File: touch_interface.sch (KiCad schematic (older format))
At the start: 18 parts, among them SW2 SW_Push, U5 ASMT-YTC2-0AA02

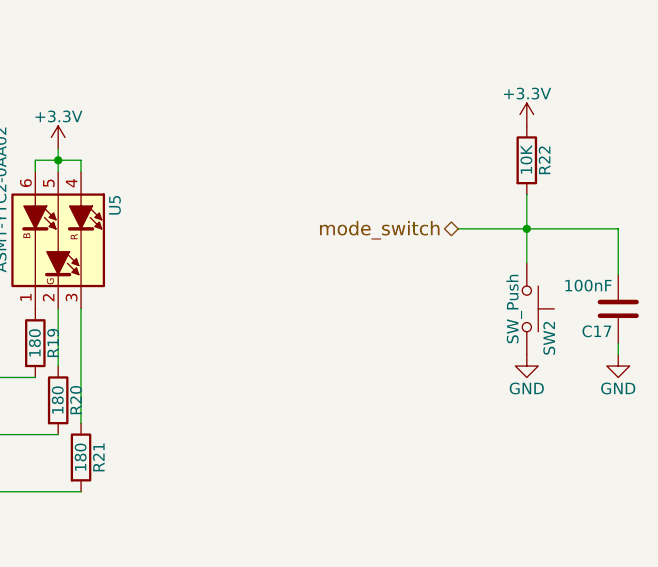
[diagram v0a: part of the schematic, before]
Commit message: Update to new soft-latching power circuit
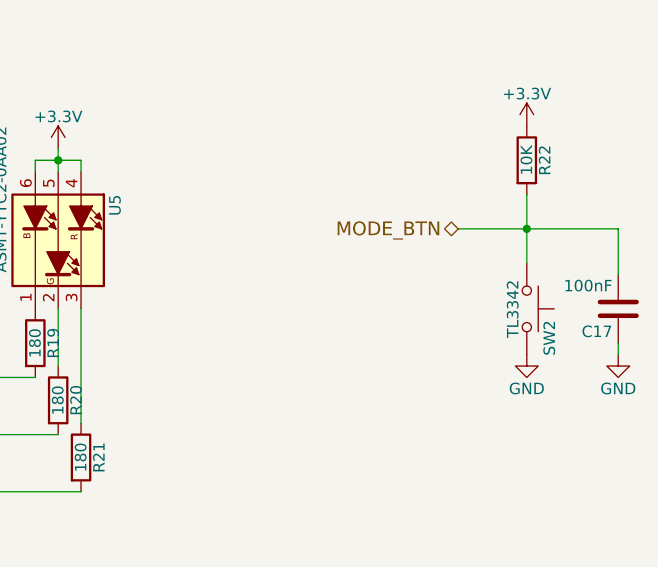
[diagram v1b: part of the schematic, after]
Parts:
- SW2: value SW_Push -> TL3342
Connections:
- net mode_switch renamed MODE_BTN
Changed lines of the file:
@@
 LED_RED
 Text HLabel 9000 2900 0    60   BiDi ~ 0
-mode_switch
+MODE_BTN
 $Comp
 L R R22
@@
 P 9300 3250
 F 0 "SW2" H 9350 3350 50  0000 L CNN
-F 1 "SW_Push" H 9300 3190 50  0000 C CNN
+F 1 "TL3342" H 9300 3190 50  0000 C CNN
 F 2 "Buttons_Switches_SMD:SW_SPST_TL3342" H 9300 3450 50  0001 C CNN
 F 3 "" H 9300 3450 50  0001 C CNN

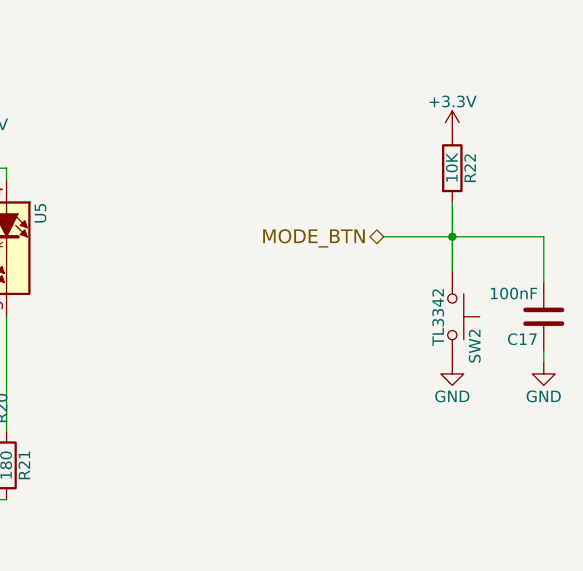
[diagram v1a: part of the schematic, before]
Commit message: attempt 1
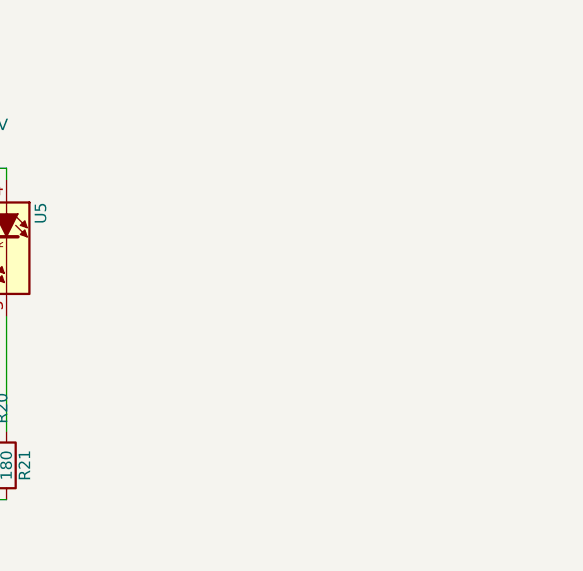
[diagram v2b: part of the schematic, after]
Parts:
- removed C17: 100nF, Capacitors_SMD:C_0603, symbol C
- removed R22: 10K, Resistors_SMD:R_0603, symbol R
- removed SW2: TL3342, Buttons_Switches_SMD:SW_SPST_TL3342, symbol SW_Push
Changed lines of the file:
@@
 Text HLabel 6650 4050 0    60   BiDi ~ 0
 LED_RED
-Text HLabel 9000 2900 0    60   BiDi ~ 0
-MODE_BTN
-$Comp
-L R R22
-U 1 1 59A90FE3
-P 9300 2600
-F 0 "R22" V 9380 2600 50  0000 C CNN
-F 1 "10K" V 9300 2600 50  0000 C CNN
-F 2 "Resistors_SMD:R_0603" V 9230 2600 50  0001 C CNN
-F 3 "" H 9300 2600 50  0001 C CNN
-	1    9300 2600
-	1    0    0    -1
-$EndComp
-$Comp
-L SW_Push SW2
-U 1 1 59A9121A
-P 9300 3250
-F 0 "SW2" H 9350 3350 50  0000 L CNN
-F 1 "TL3342" H 9300 3190 50  0000 C CNN
-F 2 "Buttons_Switches_SMD:SW_SPST_TL3342" H 9300 3450 50  0001 C CNN
-F 3 "" H 9300 3450 50  0001 C CNN
-	1    9300 3250
-	0    1    1    0
-$EndComp
-Wire Wire Line
-	9000 2900 9700 2900
-Wire Wire Line
-	9300 2750 9300 3050
-Connection ~ 9300 2900
-$Comp
-L GND #PWR034
-U 1 1 59A91325
-P 9300 3450
-F 0 "#PWR034" H 9300 3200 50  0001 C CNN
-F 1 "GND" H 9300 3300 50  0000 C CNN
-F 2 "" H 9300 3450 50  0001 C CNN
-F 3 "" H 9300 3450 50  0001 C CNN
-	1    9300 3450
-	1    0    0    -1
-$EndComp
-$Comp
-L +3.3V #PWR035
-U 1 1 59A91458
-P 9300 2450
-F 0 "#PWR035" H 9300 2300 50  0001 C CNN
-F 1 "+3.3V" H 9300 2590 50  0000 C CNN
-F 2 "" H 9300 2450 50  0001 C CNN
-F 3 "" H 9300 2450 50  0001 C CNN
-	1    9300 2450
-	1    0    0    -1
-$EndComp
-$Comp
-L C C17
-U 1 1 59A91CFD
-P 9700 3250
-F 0 "C17" H 9725 3350 50  0000 L CNN
-F 1 "100nF" H 9725 3150 50  0000 L CNN
-F 2 "Capacitors_SMD:C_0603" H 9738 3100 50  0001 C CNN
-F 3 "" H 9700 3250 50  0001 C CNN
-	1    9700 3250
-	-1   0    0    1
-$EndComp
-Wire Wire Line
-	9700 2900 9700 3100
-$Comp
-L GND #PWR036
-U 1 1 59A91F4D
-P 9700 3450
-F 0 "#PWR036" H 9700 3200 50  0001 C CNN
-F 1 "GND" H 9700 3300 50  0000 C CNN
-F 2 "" H 9700 3450 50  0001 C CNN
-F 3 "" H 9700 3450 50  0001 C CNN
-	1    9700 3450
-	1    0    0    -1
-$EndComp
-Wire Wire Line
-	9700 3400 9700 3450
 $EndSCHEMATC

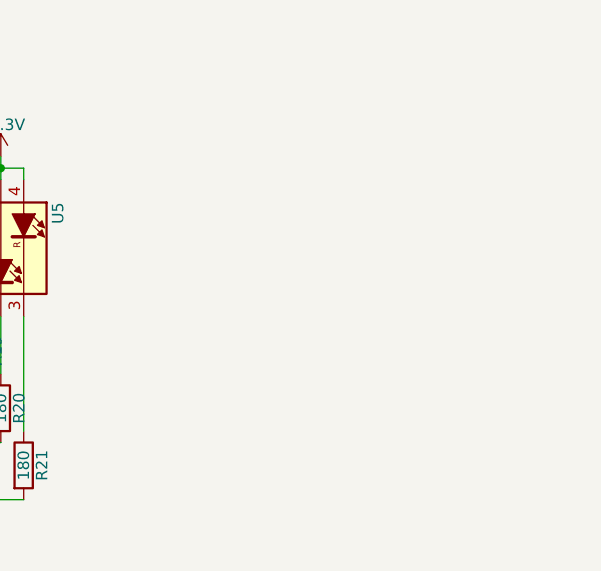
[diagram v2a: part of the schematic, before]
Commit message: Add switch footprints, add mode switch
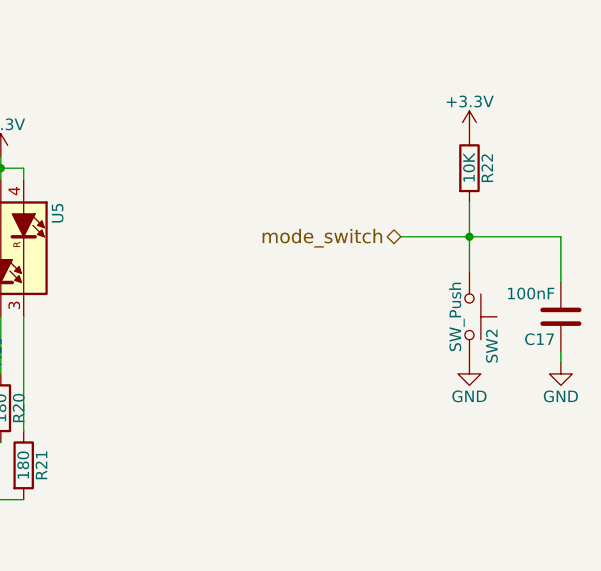
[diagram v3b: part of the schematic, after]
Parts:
- added C17: 100nF, Capacitors_SMD:C_0603, symbol C
- added R22: 10K, Resistors_SMD:R_0603, symbol R
- added SW2: SW_Push, Buttons_Switches_SMD:SW_SPST_TL3342, symbol SW_Push
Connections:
- net +3V3: now also R22.1
- net GND: now also C17.1, SW2.2
- new net mode_switch: C17.2, R22.2, SW2.1
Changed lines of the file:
@@
 Text HLabel 6650 4050 0    60   BiDi ~ 0
 LED_RED
+Text HLabel 9000 2900 0    60   BiDi ~ 0
+mode_switch
+$Comp
+L R R22
+U 1 1 59A90FE3
+P 9300 2600
+F 0 "R22" V 9380 2600 50  0000 C CNN
+F 1 "10K" V 9300 2600 50  0000 C CNN
+F 2 "Resistors_SMD:R_0603" V 9230 2600 50  0001 C CNN
+F 3 "" H 9300 2600 50  0001 C CNN
+	1    9300 2600
+	1    0    0    -1
+$EndComp
+$Comp
+L SW_Push SW2
+U 1 1 59A9121A
+P 9300 3250
+F 0 "SW2" H 9350 3350 50  0000 L CNN
+F 1 "SW_Push" H 9300 3190 50  0000 C CNN
+F 2 "Buttons_Switches_SMD:SW_SPST_TL3342" H 9300 3450 50  0001 C CNN
+F 3 "" H 9300 3450 50  0001 C CNN
+	1    9300 3250
+	0    1    1    0
+$EndComp
+Wire Wire Line
+	9000 2900 9700 2900
+Wire Wire Line
+	9300 2750 9300 3050
+Connection ~ 9300 2900
+$Comp
+L GND #PWR034
+U 1 1 59A91325
+P 9300 3450
+F 0 "#PWR034" H 9300 3200 50  0001 C CNN
+F 1 "GND" H 9300 3300 50  0000 C CNN
+F 2 "" H 9300 3450 50  0001 C CNN
+F 3 "" H 9300 3450 50  0001 C CNN
+	1    9300 3450
+	1    0    0    -1
+$EndComp
+$Comp
+L +3.3V #PWR035
+U 1 1 59A91458
+P 9300 2450
+F 0 "#PWR035" H 9300 2300 50  0001 C CNN
+F 1 "+3.3V" H 9300 2590 50  0000 C CNN
+F 2 "" H 9300 2450 50  0001 C CNN
+F 3 "" H 9300 2450 50  0001 C CNN
+	1    9300 2450
+	1    0    0    -1
+$EndComp
+$Comp
+L C C17
+U 1 1 59A91CFD
+P 9700 3250
+F 0 "C17" H 9725 3350 50  0000 L CNN
+F 1 "100nF" H 9725 3150 50  0000 L CNN
+F 2 "Capacitors_SMD:C_0603" H 9738 3100 50  0001 C CNN
+F 3 "" H 9700 3250 50  0001 C CNN
+	1    9700 3250
+	-1   0    0    1
+$EndComp
+Wire Wire Line
+	9700 2900 9700 3100
+$Comp
+L GND #PWR036
+U 1 1 59A91F4D
+P 9700 3450
+F 0 "#PWR036" H 9700 3200 50  0001 C CNN
+F 1 "GND" H 9700 3300 50  0000 C CNN
+F 2 "" H 9700 3450 50  0001 C CNN
+F 3 "" H 9700 3450 50  0001 C CNN
+	1    9700 3450
+	1    0    0    -1
+$EndComp
+Wire Wire Line
+	9700 3400 9700 3450
 $EndSCHEMATC
